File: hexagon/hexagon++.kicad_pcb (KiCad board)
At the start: 2 copper layers, 97.7 x 86.5 mm, 27 parts, among them J1 Conn_01x05_Pin, J2 Conn_01x05_Pin, J3 Conn_01x05_Pin, J4 Conn_01x05_Pin, J5 Conn_01x05_Pin, J6 Conn_01x05_Pin

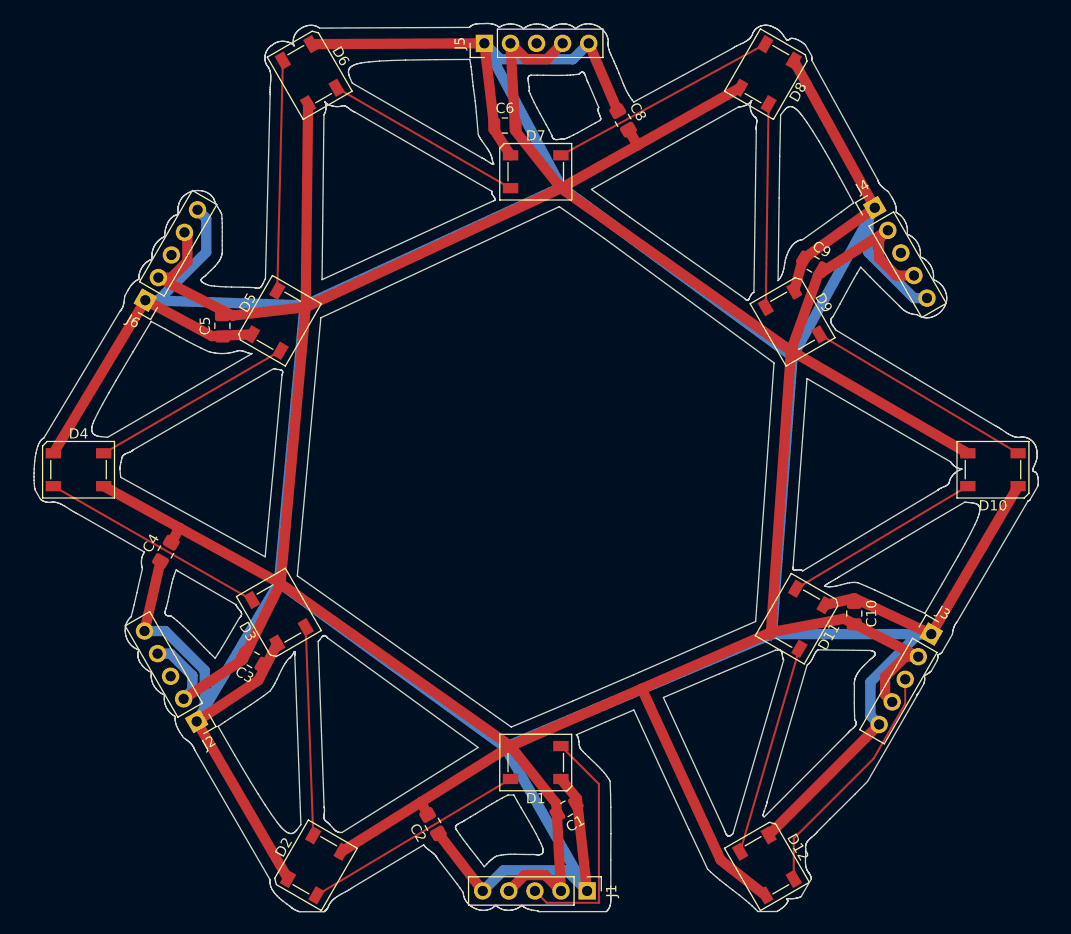
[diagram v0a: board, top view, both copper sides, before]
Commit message: great success!
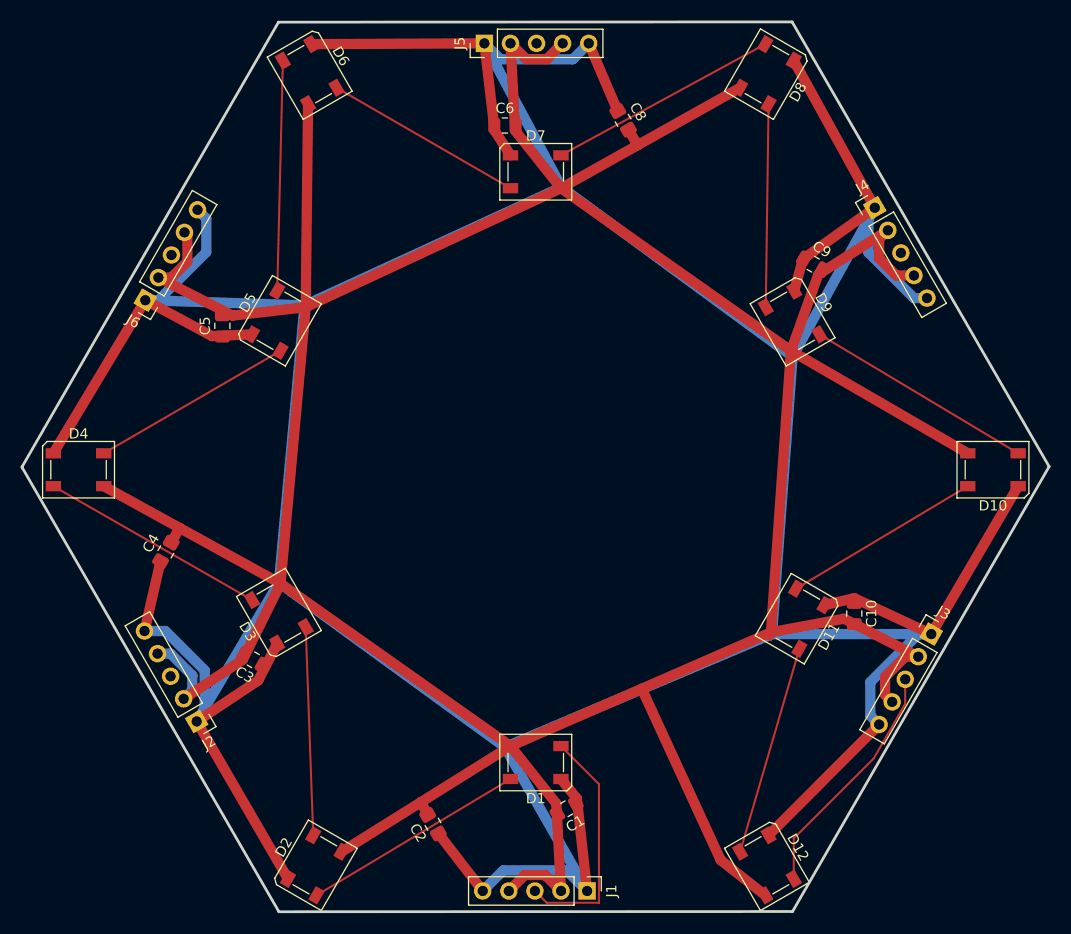
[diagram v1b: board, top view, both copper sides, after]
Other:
- board size 97.7 x 86.5 mm -> 100 x 86.6 mm
